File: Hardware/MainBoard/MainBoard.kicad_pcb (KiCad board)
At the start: 2 copper layers, 70 x 71 mm, 13 parts, among them J1 Conn_02x20_Odd_Even, J5 USB_B_Micro, U3 LD1117ASTR

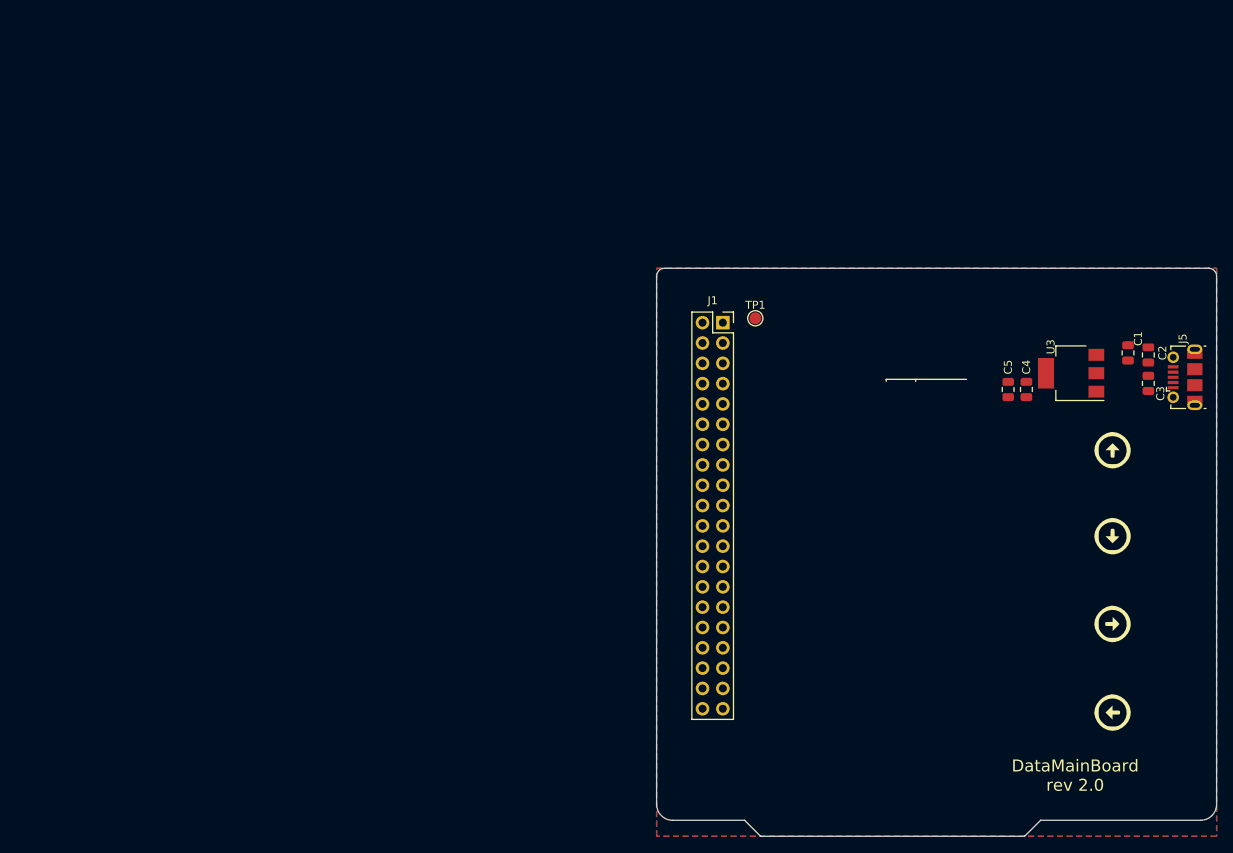
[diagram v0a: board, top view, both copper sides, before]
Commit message: draft of mainboard
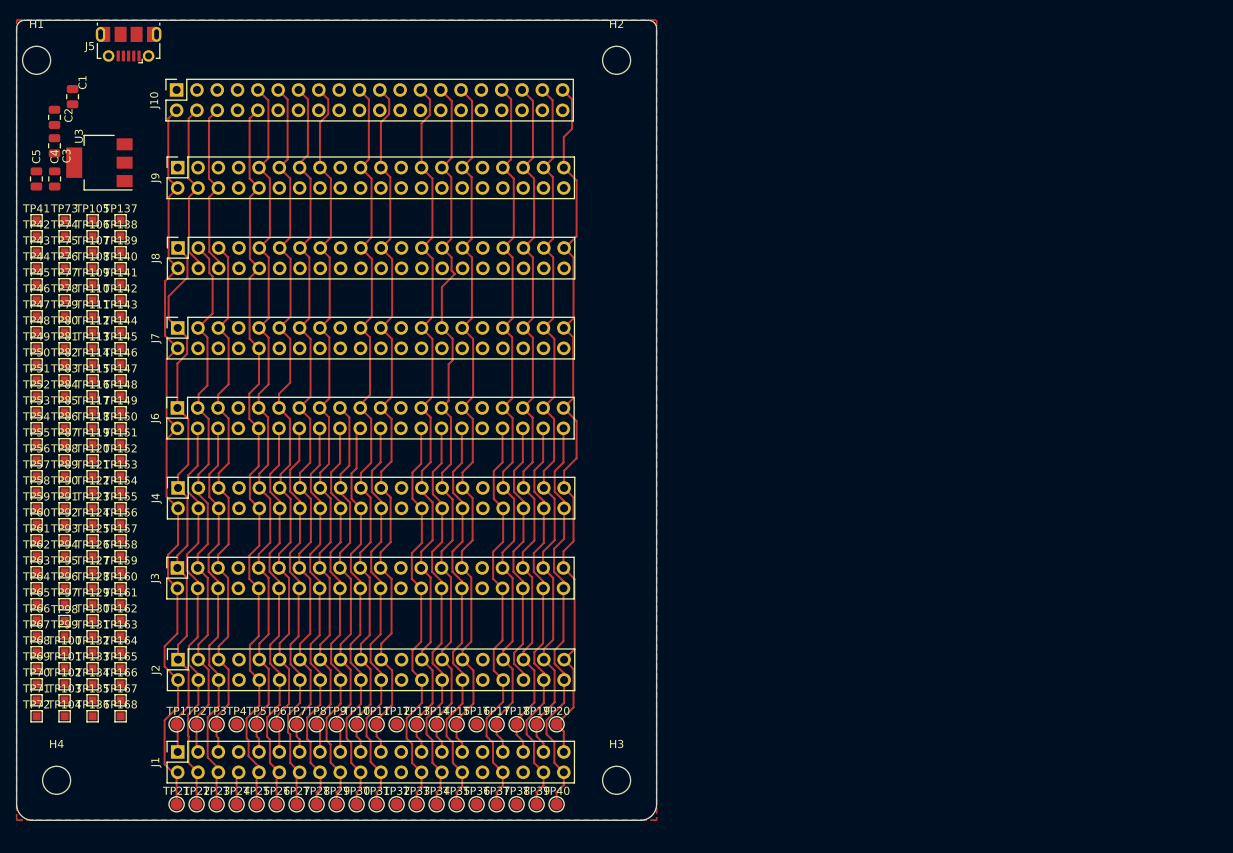
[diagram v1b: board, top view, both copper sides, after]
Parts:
- removed G***: LOGO, MainBoard:arrow-right-circle-line
- removed G***: LOGO, MainBoard:arrow-up-circle-line
- removed G***: LOGO, MainBoard:arrow-left-circle-line
- removed G***: LOGO, MainBoard:arrow-down-circle-line
- added H1: MountingHole, MountingHole:MountingHole_3.5mm, F.Cu at (52.5, 25.0)
- added H2: MountingHole, MountingHole:MountingHole_3.5mm, F.Cu at (125.0, 25.0)
- added H3: MountingHole, MountingHole:MountingHole_3.5mm, F.Cu at (125.0, 115.0)
- added H4: MountingHole, MountingHole:MountingHole_3.5mm, F.Cu at (55.0, 115.0)
- added J10: Conn_02x20_Odd_Even, Connector_PinSocket_2.54mm:PinSocket_2x20_P2.54mm_Vertical, F.Cu at (70.0, 28.7)
- added J2: Conn_02x20_Odd_Even, Connector_PinSocket_2.54mm:PinSocket_2x20_P2.54mm_Vertical, F.Cu at (70.2, 99.9)
- added J3: Conn_02x20_Odd_Even, Connector_PinSocket_2.54mm:PinSocket_2x20_P2.54mm_Vertical, F.Cu at (70.1, 88.5)
- added J4: Conn_02x20_Odd_Even, Connector_PinSocket_2.54mm:PinSocket_2x20_P2.54mm_Vertical, F.Cu at (70.2, 78.5)
- added J6: Conn_02x20_Odd_Even, Connector_PinSocket_2.54mm:PinSocket_2x20_P2.54mm_Vertical, F.Cu at (70.1, 68.5)
- added J7: Conn_02x20_Odd_Even, Connector_PinSocket_2.54mm:PinSocket_2x20_P2.54mm_Vertical, F.Cu at (70.1, 58.5)
- added J8: Conn_02x20_Odd_Even, Connector_PinSocket_2.54mm:PinSocket_2x20_P2.54mm_Vertical, F.Cu at (70.2, 48.5)
- added J9: Conn_02x20_Odd_Even, Connector_PinSocket_2.54mm:PinSocket_2x20_P2.54mm_Vertical, F.Cu at (70.1, 38.4)
- added TP10: TestPoint, TestPoint:TestPoint_Pad_D1.5mm, F.Cu at (92.5, 108.0)
- added TP100: TestPoint, TestPoint:TestPoint_Pad_1.0x1.0mm, F.Cu at (56.0, 99.0)
- added TP101: TestPoint, TestPoint:TestPoint_Pad_1.0x1.0mm, F.Cu at (56.0, 101.0)
- added TP102: TestPoint, TestPoint:TestPoint_Pad_1.0x1.0mm, F.Cu at (56.0, 103.0)
- added TP103: TestPoint, TestPoint:TestPoint_Pad_1.0x1.0mm, F.Cu at (56.0, 105.0)
- added TP104: TestPoint, TestPoint:TestPoint_Pad_1.0x1.0mm, F.Cu at (56.0, 107.0)
- added TP105: TestPoint, TestPoint:TestPoint_Pad_1.0x1.0mm, F.Cu at (59.5, 45.0)
- added TP106: TestPoint, TestPoint:TestPoint_Pad_1.0x1.0mm, F.Cu at (59.5, 47.0)
- added TP107: TestPoint, TestPoint:TestPoint_Pad_1.0x1.0mm, F.Cu at (59.5, 49.0)
- added TP108: TestPoint, TestPoint:TestPoint_Pad_1.0x1.0mm, F.Cu at (59.5, 51.0)
- added TP109: TestPoint, TestPoint:TestPoint_Pad_1.0x1.0mm, F.Cu at (59.5, 53.0)
- added TP11: TestPoint, TestPoint:TestPoint_Pad_D1.5mm, F.Cu at (95.0, 108.0)
- added TP110: TestPoint, TestPoint:TestPoint_Pad_1.0x1.0mm, F.Cu at (59.5, 55.0)
- added TP111: TestPoint, TestPoint:TestPoint_Pad_1.0x1.0mm, F.Cu at (59.5, 57.0)
- added TP112: TestPoint, TestPoint:TestPoint_Pad_1.0x1.0mm, F.Cu at (59.5, 59.0)
- added TP113: TestPoint, TestPoint:TestPoint_Pad_1.0x1.0mm, F.Cu at (59.5, 61.0)
- added TP114: TestPoint, TestPoint:TestPoint_Pad_1.0x1.0mm, F.Cu at (59.5, 63.0)
- added TP115: TestPoint, TestPoint:TestPoint_Pad_1.0x1.0mm, F.Cu at (59.5, 65.0)
- added TP116: TestPoint, TestPoint:TestPoint_Pad_1.0x1.0mm, F.Cu at (59.5, 67.0)
- added TP117: TestPoint, TestPoint:TestPoint_Pad_1.0x1.0mm, F.Cu at (59.5, 69.0)
- added TP118: TestPoint, TestPoint:TestPoint_Pad_1.0x1.0mm, F.Cu at (59.5, 71.0)
- added TP119: TestPoint, TestPoint:TestPoint_Pad_1.0x1.0mm, F.Cu at (59.5, 73.0)
- added TP12: TestPoint, TestPoint:TestPoint_Pad_D1.5mm, F.Cu at (97.5, 108.0)
- added TP120: TestPoint, TestPoint:TestPoint_Pad_1.0x1.0mm, F.Cu at (59.5, 75.0)
- added TP121: TestPoint, TestPoint:TestPoint_Pad_1.0x1.0mm, F.Cu at (59.5, 77.0)
- added TP122: TestPoint, TestPoint:TestPoint_Pad_1.0x1.0mm, F.Cu at (59.5, 79.0)
- added TP123: TestPoint, TestPoint:TestPoint_Pad_1.0x1.0mm, F.Cu at (59.5, 81.0)
- added TP124: TestPoint, TestPoint:TestPoint_Pad_1.0x1.0mm, F.Cu at (59.5, 83.0)
- added TP125: TestPoint, TestPoint:TestPoint_Pad_1.0x1.0mm, F.Cu at (59.5, 85.0)
- added TP126: TestPoint, TestPoint:TestPoint_Pad_1.0x1.0mm, F.Cu at (59.5, 87.0)
- added TP127: TestPoint, TestPoint:TestPoint_Pad_1.0x1.0mm, F.Cu at (59.5, 89.0)
- added TP128: TestPoint, TestPoint:TestPoint_Pad_1.0x1.0mm, F.Cu at (59.5, 91.0)
- added TP129: TestPoint, TestPoint:TestPoint_Pad_1.0x1.0mm, F.Cu at (59.5, 93.0)
- added TP13: TestPoint, TestPoint:TestPoint_Pad_D1.5mm, F.Cu at (100.0, 108.0)
- added TP130: TestPoint, TestPoint:TestPoint_Pad_1.0x1.0mm, F.Cu at (59.5, 95.0)
- added TP131: TestPoint, TestPoint:TestPoint_Pad_1.0x1.0mm, F.Cu at (59.5, 97.0)
- added TP132: TestPoint, TestPoint:TestPoint_Pad_1.0x1.0mm, F.Cu at (59.5, 99.0)
- added TP133: TestPoint, TestPoint:TestPoint_Pad_1.0x1.0mm, F.Cu at (59.5, 101.0)
- added TP134: TestPoint, TestPoint:TestPoint_Pad_1.0x1.0mm, F.Cu at (59.5, 103.0)
- added TP135: TestPoint, TestPoint:TestPoint_Pad_1.0x1.0mm, F.Cu at (59.5, 105.0)
- added TP136: TestPoint, TestPoint:TestPoint_Pad_1.0x1.0mm, F.Cu at (59.5, 107.0)
- added TP137: TestPoint, TestPoint:TestPoint_Pad_1.0x1.0mm, F.Cu at (63.0, 45.0)
- added TP138: TestPoint, TestPoint:TestPoint_Pad_1.0x1.0mm, F.Cu at (63.0, 47.0)
- added TP139: TestPoint, TestPoint:TestPoint_Pad_1.0x1.0mm, F.Cu at (63.0, 49.0)
- added TP14: TestPoint, TestPoint:TestPoint_Pad_D1.5mm, F.Cu at (102.5, 108.0)
- added TP140: TestPoint, TestPoint:TestPoint_Pad_1.0x1.0mm, F.Cu at (63.0, 51.0)
- added TP141: TestPoint, TestPoint:TestPoint_Pad_1.0x1.0mm, F.Cu at (63.0, 53.0)
- added TP142: TestPoint, TestPoint:TestPoint_Pad_1.0x1.0mm, F.Cu at (63.0, 55.0)
- added TP143: TestPoint, TestPoint:TestPoint_Pad_1.0x1.0mm, F.Cu at (63.0, 57.0)
- added TP144: TestPoint, TestPoint:TestPoint_Pad_1.0x1.0mm, F.Cu at (63.0, 59.0)
- added TP145: TestPoint, TestPoint:TestPoint_Pad_1.0x1.0mm, F.Cu at (63.0, 61.0)
- added TP146: TestPoint, TestPoint:TestPoint_Pad_1.0x1.0mm, F.Cu at (63.0, 63.0)
- added TP147: TestPoint, TestPoint:TestPoint_Pad_1.0x1.0mm, F.Cu at (63.0, 65.0)
- added TP148: TestPoint, TestPoint:TestPoint_Pad_1.0x1.0mm, F.Cu at (63.0, 67.0)
- added TP149: TestPoint, TestPoint:TestPoint_Pad_1.0x1.0mm, F.Cu at (63.0, 69.0)
- added TP15: TestPoint, TestPoint:TestPoint_Pad_D1.5mm, F.Cu at (105.0, 108.0)
- added TP150: TestPoint, TestPoint:TestPoint_Pad_1.0x1.0mm, F.Cu at (63.0, 71.0)
- added TP151: TestPoint, TestPoint:TestPoint_Pad_1.0x1.0mm, F.Cu at (63.0, 73.0)
- added TP152: TestPoint, TestPoint:TestPoint_Pad_1.0x1.0mm, F.Cu at (63.0, 75.0)
- added TP153: TestPoint, TestPoint:TestPoint_Pad_1.0x1.0mm, F.Cu at (63.0, 77.0)
- added TP154: TestPoint, TestPoint:TestPoint_Pad_1.0x1.0mm, F.Cu at (63.0, 79.0)
- added TP155: TestPoint, TestPoint:TestPoint_Pad_1.0x1.0mm, F.Cu at (63.0, 81.0)
- added TP156: TestPoint, TestPoint:TestPoint_Pad_1.0x1.0mm, F.Cu at (63.0, 83.0)
- added TP157: TestPoint, TestPoint:TestPoint_Pad_1.0x1.0mm, F.Cu at (63.0, 85.0)
- added TP158: TestPoint, TestPoint:TestPoint_Pad_1.0x1.0mm, F.Cu at (63.0, 87.0)
- added TP159: TestPoint, TestPoint:TestPoint_Pad_1.0x1.0mm, F.Cu at (63.0, 89.0)
- added TP16: TestPoint, TestPoint:TestPoint_Pad_D1.5mm, F.Cu at (107.5, 108.0)
- added TP160: TestPoint, TestPoint:TestPoint_Pad_1.0x1.0mm, F.Cu at (63.0, 91.0)
- added TP161: TestPoint, TestPoint:TestPoint_Pad_1.0x1.0mm, F.Cu at (63.0, 93.0)
- added TP162: TestPoint, TestPoint:TestPoint_Pad_1.0x1.0mm, F.Cu at (63.0, 95.0)
- added TP163: TestPoint, TestPoint:TestPoint_Pad_1.0x1.0mm, F.Cu at (63.0, 97.0)
- added TP164: TestPoint, TestPoint:TestPoint_Pad_1.0x1.0mm, F.Cu at (63.0, 99.0)
- added TP165: TestPoint, TestPoint:TestPoint_Pad_1.0x1.0mm, F.Cu at (63.0, 101.0)
- added TP166: TestPoint, TestPoint:TestPoint_Pad_1.0x1.0mm, F.Cu at (63.0, 103.0)
- added TP167: TestPoint, TestPoint:TestPoint_Pad_1.0x1.0mm, F.Cu at (63.0, 105.0)
- added TP168: TestPoint, TestPoint:TestPoint_Pad_1.0x1.0mm, F.Cu at (63.0, 107.0)
- added TP17: TestPoint, TestPoint:TestPoint_Pad_D1.5mm, F.Cu at (110.0, 108.0)
- added TP18: TestPoint, TestPoint:TestPoint_Pad_D1.5mm, F.Cu at (112.5, 108.0)
- added TP19: TestPoint, TestPoint:TestPoint_Pad_D1.5mm, F.Cu at (115.0, 108.0)
- added TP2: TestPoint, TestPoint:TestPoint_Pad_D1.5mm, F.Cu at (72.5, 108.0)
- added TP20: TestPoint, TestPoint:TestPoint_Pad_D1.5mm, F.Cu at (117.5, 108.0)
- added TP21: TestPoint, TestPoint:TestPoint_Pad_D1.5mm, F.Cu at (70.0, 118.0)
- added TP22: TestPoint, TestPoint:TestPoint_Pad_D1.5mm, F.Cu at (72.5, 118.0)
- added TP23: TestPoint, TestPoint:TestPoint_Pad_D1.5mm, F.Cu at (75.0, 118.0)
- added TP24: TestPoint, TestPoint:TestPoint_Pad_D1.5mm, F.Cu at (77.5, 118.0)
- added TP25: TestPoint, TestPoint:TestPoint_Pad_D1.5mm, F.Cu at (80.0, 118.0)
- added TP26: TestPoint, TestPoint:TestPoint_Pad_D1.5mm, F.Cu at (82.5, 118.0)
- added TP27: TestPoint, TestPoint:TestPoint_Pad_D1.5mm, F.Cu at (85.0, 118.0)
- added TP28: TestPoint, TestPoint:TestPoint_Pad_D1.5mm, F.Cu at (87.5, 118.0)
- added TP29: TestPoint, TestPoint:TestPoint_Pad_D1.5mm, F.Cu at (90.0, 118.0)
- added TP3: TestPoint, TestPoint:TestPoint_Pad_D1.5mm, F.Cu at (75.0, 108.0)
- added TP30: TestPoint, TestPoint:TestPoint_Pad_D1.5mm, F.Cu at (92.5, 118.0)
- added TP31: TestPoint, TestPoint:TestPoint_Pad_D1.5mm, F.Cu at (95.0, 118.0)
- added TP32: TestPoint, TestPoint:TestPoint_Pad_D1.5mm, F.Cu at (97.5, 118.0)
- added TP33: TestPoint, TestPoint:TestPoint_Pad_D1.5mm, F.Cu at (100.0, 118.0)
- added TP34: TestPoint, TestPoint:TestPoint_Pad_D1.5mm, F.Cu at (102.5, 118.0)
- added TP35: TestPoint, TestPoint:TestPoint_Pad_D1.5mm, F.Cu at (105.0, 118.0)
- added TP36: TestPoint, TestPoint:TestPoint_Pad_D1.5mm, F.Cu at (107.5, 118.0)
- added TP37: TestPoint, TestPoint:TestPoint_Pad_D1.5mm, F.Cu at (110.0, 118.0)
- added TP38: TestPoint, TestPoint:TestPoint_Pad_D1.5mm, F.Cu at (112.5, 118.0)
- added TP39: TestPoint, TestPoint:TestPoint_Pad_D1.5mm, F.Cu at (115.0, 118.0)
- added TP4: TestPoint, TestPoint:TestPoint_Pad_D1.5mm, F.Cu at (77.5, 108.0)
- added TP40: TestPoint, TestPoint:TestPoint_Pad_D1.5mm, F.Cu at (117.5, 118.0)
- added TP41: TestPoint, TestPoint:TestPoint_Pad_1.0x1.0mm, F.Cu at (52.5, 45.0)
- added TP42: TestPoint, TestPoint:TestPoint_Pad_1.0x1.0mm, F.Cu at (52.5, 47.0)
- added TP43: TestPoint, TestPoint:TestPoint_Pad_1.0x1.0mm, F.Cu at (52.5, 49.0)
- added TP44: TestPoint, TestPoint:TestPoint_Pad_1.0x1.0mm, F.Cu at (52.5, 51.0)
- added TP45: TestPoint, TestPoint:TestPoint_Pad_1.0x1.0mm, F.Cu at (52.5, 53.0)
- added TP46: TestPoint, TestPoint:TestPoint_Pad_1.0x1.0mm, F.Cu at (52.5, 55.0)
- added TP47: TestPoint, TestPoint:TestPoint_Pad_1.0x1.0mm, F.Cu at (52.5, 57.0)
- added TP48: TestPoint, TestPoint:TestPoint_Pad_1.0x1.0mm, F.Cu at (52.5, 59.0)
- added TP49: TestPoint, TestPoint:TestPoint_Pad_1.0x1.0mm, F.Cu at (52.5, 61.0)
- added TP5: TestPoint, TestPoint:TestPoint_Pad_D1.5mm, F.Cu at (80.0, 108.0)
- added TP50: TestPoint, TestPoint:TestPoint_Pad_1.0x1.0mm, F.Cu at (52.5, 63.0)
- added TP51: TestPoint, TestPoint:TestPoint_Pad_1.0x1.0mm, F.Cu at (52.5, 65.0)
- added TP52: TestPoint, TestPoint:TestPoint_Pad_1.0x1.0mm, F.Cu at (52.5, 67.0)
- added TP53: TestPoint, TestPoint:TestPoint_Pad_1.0x1.0mm, F.Cu at (52.5, 69.0)
- added TP54: TestPoint, TestPoint:TestPoint_Pad_1.0x1.0mm, F.Cu at (52.5, 71.0)
- added TP55: TestPoint, TestPoint:TestPoint_Pad_1.0x1.0mm, F.Cu at (52.5, 73.0)
- added TP56: TestPoint, TestPoint:TestPoint_Pad_1.0x1.0mm, F.Cu at (52.5, 75.0)
- added TP57: TestPoint, TestPoint:TestPoint_Pad_1.0x1.0mm, F.Cu at (52.5, 77.0)
- added TP58: TestPoint, TestPoint:TestPoint_Pad_1.0x1.0mm, F.Cu at (52.5, 79.0)
- added TP59: TestPoint, TestPoint:TestPoint_Pad_1.0x1.0mm, F.Cu at (52.5, 81.0)
- added TP6: TestPoint, TestPoint:TestPoint_Pad_D1.5mm, F.Cu at (82.5, 108.0)
- added TP60: TestPoint, TestPoint:TestPoint_Pad_1.0x1.0mm, F.Cu at (52.5, 83.0)
- added TP61: TestPoint, TestPoint:TestPoint_Pad_1.0x1.0mm, F.Cu at (52.5, 85.0)
- added TP62: TestPoint, TestPoint:TestPoint_Pad_1.0x1.0mm, F.Cu at (52.5, 87.0)
- added TP63: TestPoint, TestPoint:TestPoint_Pad_1.0x1.0mm, F.Cu at (52.5, 89.0)
- added TP64: TestPoint, TestPoint:TestPoint_Pad_1.0x1.0mm, F.Cu at (52.5, 91.0)
- added TP65: TestPoint, TestPoint:TestPoint_Pad_1.0x1.0mm, F.Cu at (52.5, 93.0)
- added TP66: TestPoint, TestPoint:TestPoint_Pad_1.0x1.0mm, F.Cu at (52.5, 95.0)
- added TP67: TestPoint, TestPoint:TestPoint_Pad_1.0x1.0mm, F.Cu at (52.5, 97.0)
- added TP68: TestPoint, TestPoint:TestPoint_Pad_1.0x1.0mm, F.Cu at (52.5, 99.0)
- added TP69: TestPoint, TestPoint:TestPoint_Pad_1.0x1.0mm, F.Cu at (52.5, 101.0)
- added TP7: TestPoint, TestPoint:TestPoint_Pad_D1.5mm, F.Cu at (85.0, 108.0)
- added TP70: TestPoint, TestPoint:TestPoint_Pad_1.0x1.0mm, F.Cu at (52.5, 103.0)
- added TP71: TestPoint, TestPoint:TestPoint_Pad_1.0x1.0mm, F.Cu at (52.5, 105.0)
- added TP72: TestPoint, TestPoint:TestPoint_Pad_1.0x1.0mm, F.Cu at (52.5, 107.0)
- added TP73: TestPoint, TestPoint:TestPoint_Pad_1.0x1.0mm, F.Cu at (56.0, 45.0)
- added TP74: TestPoint, TestPoint:TestPoint_Pad_1.0x1.0mm, F.Cu at (56.0, 47.0)
- added TP75: TestPoint, TestPoint:TestPoint_Pad_1.0x1.0mm, F.Cu at (56.0, 49.0)
- added TP76: TestPoint, TestPoint:TestPoint_Pad_1.0x1.0mm, F.Cu at (56.0, 51.0)
- added TP77: TestPoint, TestPoint:TestPoint_Pad_1.0x1.0mm, F.Cu at (56.0, 53.0)
- added TP78: TestPoint, TestPoint:TestPoint_Pad_1.0x1.0mm, F.Cu at (56.0, 55.0)
- added TP79: TestPoint, TestPoint:TestPoint_Pad_1.0x1.0mm, F.Cu at (56.0, 57.0)
- added TP8: TestPoint, TestPoint:TestPoint_Pad_D1.5mm, F.Cu at (87.5, 108.0)
- added TP80: TestPoint, TestPoint:TestPoint_Pad_1.0x1.0mm, F.Cu at (56.0, 59.0)
- added TP81: TestPoint, TestPoint:TestPoint_Pad_1.0x1.0mm, F.Cu at (56.0, 61.0)
- added TP82: TestPoint, TestPoint:TestPoint_Pad_1.0x1.0mm, F.Cu at (56.0, 63.0)
- added TP83: TestPoint, TestPoint:TestPoint_Pad_1.0x1.0mm, F.Cu at (56.0, 65.0)
- added TP84: TestPoint, TestPoint:TestPoint_Pad_1.0x1.0mm, F.Cu at (56.0, 67.0)
- added TP85: TestPoint, TestPoint:TestPoint_Pad_1.0x1.0mm, F.Cu at (56.0, 69.0)
- added TP86: TestPoint, TestPoint:TestPoint_Pad_1.0x1.0mm, F.Cu at (56.0, 71.0)
- added TP87: TestPoint, TestPoint:TestPoint_Pad_1.0x1.0mm, F.Cu at (56.0, 73.0)
- added TP88: TestPoint, TestPoint:TestPoint_Pad_1.0x1.0mm, F.Cu at (56.0, 75.0)
- added TP89: TestPoint, TestPoint:TestPoint_Pad_1.0x1.0mm, F.Cu at (56.0, 77.0)
- added TP9: TestPoint, TestPoint:TestPoint_Pad_D1.5mm, F.Cu at (90.0, 108.0)
- added TP90: TestPoint, TestPoint:TestPoint_Pad_1.0x1.0mm, F.Cu at (56.0, 79.0)
- added TP91: TestPoint, TestPoint:TestPoint_Pad_1.0x1.0mm, F.Cu at (56.0, 81.0)
- added TP92: TestPoint, TestPoint:TestPoint_Pad_1.0x1.0mm, F.Cu at (56.0, 83.0)
- added TP93: TestPoint, TestPoint:TestPoint_Pad_1.0x1.0mm, F.Cu at (56.0, 85.0)
- added TP94: TestPoint, TestPoint:TestPoint_Pad_1.0x1.0mm, F.Cu at (56.0, 87.0)
- added TP95: TestPoint, TestPoint:TestPoint_Pad_1.0x1.0mm, F.Cu at (56.0, 89.0)
- added TP96: TestPoint, TestPoint:TestPoint_Pad_1.0x1.0mm, F.Cu at (56.0, 91.0)
- added TP97: TestPoint, TestPoint:TestPoint_Pad_1.0x1.0mm, F.Cu at (56.0, 93.0)
- added TP98: TestPoint, TestPoint:TestPoint_Pad_1.0x1.0mm, F.Cu at (56.0, 95.1)
- added TP99: TestPoint, TestPoint:TestPoint_Pad_1.0x1.0mm, F.Cu at (56.0, 97.0)
- moved C2 139.9 mm to (54.7, 32.1)
- moved C3 139.9 mm to (54.7, 35.7)
- moved J5 138.4 mm to (64.0, 23.0), turned to 180 degrees
- moved C1 135.8 mm to (57.0, 29.6)
- moved C4 124.3 mm to (54.8, 39.8)
- moved C5 124.3 mm to (52.5, 39.8)
- moved U3 124.3 mm to (60.4, 37.8)
- moved TP1 88.4 mm to (70.0, 108.0)
- moved J1 86.7 mm to (70.1, 111.5), turned to 90 degrees
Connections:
- TP1 pad 1: unconnected-(TP1-Pad1) -> -5V
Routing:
- net 5V: track 0.00 -> 96.4 mm
- net GPIO2: track 0.00 -> 94.9 mm
- net UART2_TX: track 0.00 -> 92.2 mm
- net UART1_TX: track 0.00 -> 92.0 mm
- net ANALOG3: track 0.00 -> 91.9 mm
- net SPI_MISO: track 0.00 -> 91.8 mm
- net SPI_CS2: track 0.00 -> 91.8 mm
- net SPI_SCLK: track 0.00 -> 91.7 mm
- net I2C_SCL: track 0.00 -> 91.7 mm
- net GPIO5: track 0.00 -> 91.7 mm
- net GPIO3: track 0.00 -> 91.6 mm
- net ANALOG1: track 0.00 -> 91.6 mm
- net GPIO11: track 0.00 -> 91.4 mm
- net GPIO7: track 0.00 -> 91.2 mm
- net GPIO1: track 0.00 -> 91.2 mm
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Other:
- board size 70 x 71 mm -> 80 x 100 mm
- board text added: "MainBoard rev 4.0"
- board text removed: "AVDD U5V"
- board text removed: "DataMainBoard rev 2.0"
- board text removed: "FP11-BOOT0 GND"
- board text removed: "GND GND"
- board text removed: "GND NC"
- board text removed: "NC IOREF"
- board text removed: "NC NC"
- board text removed: "PA10 PC4"
- board text removed: "PA13 RESET"
- board text removed: "PA14 +3V3"
- board text removed: "PA15 +5V"
- board text removed: "PA2 NC"
- board text removed: "PA3 NC"
- board text removed: "PA5 PA12"
- board text removed: "PA6 PA11"
- board text removed: "PA7 PB12"
- board text removed: "PA8 PB1"
- board text removed: "PA9 PB2"
- board text removed: "PB10 PB15"
- board text removed: "PB3 AGND"
- board text removed: "PB4 PB14"
- board text removed: "PB5 PB13"
- board text removed: "PB6 PB11"
- board text removed: "PB7 GND"
- board text removed: "PB8 PC6"
- board text removed: "PB9 PC5"
- board text removed: "PC10 PC11"
- board text removed: "PC12 PD2"
- board text removed: "PC13 VIN"
- board text removed: "PC14 NC"
- board text removed: "PC15 PA0"
- board text removed: "PC2 PC1"
- board text removed: "PC3 PC0"
- board text removed: "PC7 GND"
- board text removed: "PC9 PC8"
- board text removed: "PF0 PA1"
- board text removed: "PF1 PA4"
- board text removed: "VBAT PB0"
- board text removed: "VDD E5V"
